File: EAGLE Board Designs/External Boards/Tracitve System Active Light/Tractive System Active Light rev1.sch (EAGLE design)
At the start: 25 parts, among them X1 CONNECTOR-4NANO-FIT-VERTICAL-4

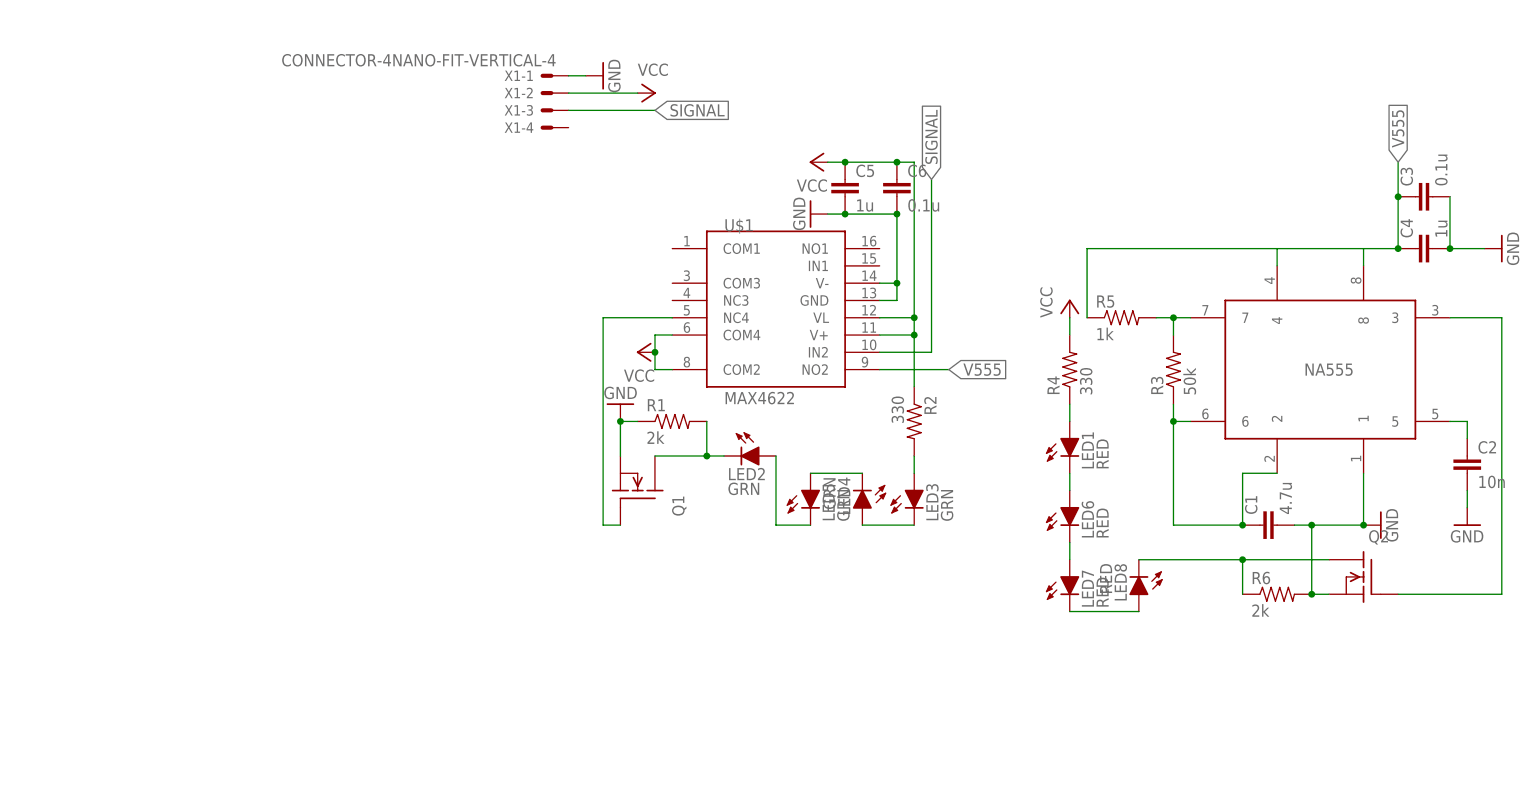
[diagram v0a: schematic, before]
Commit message: Later version of TSAL schematic and board
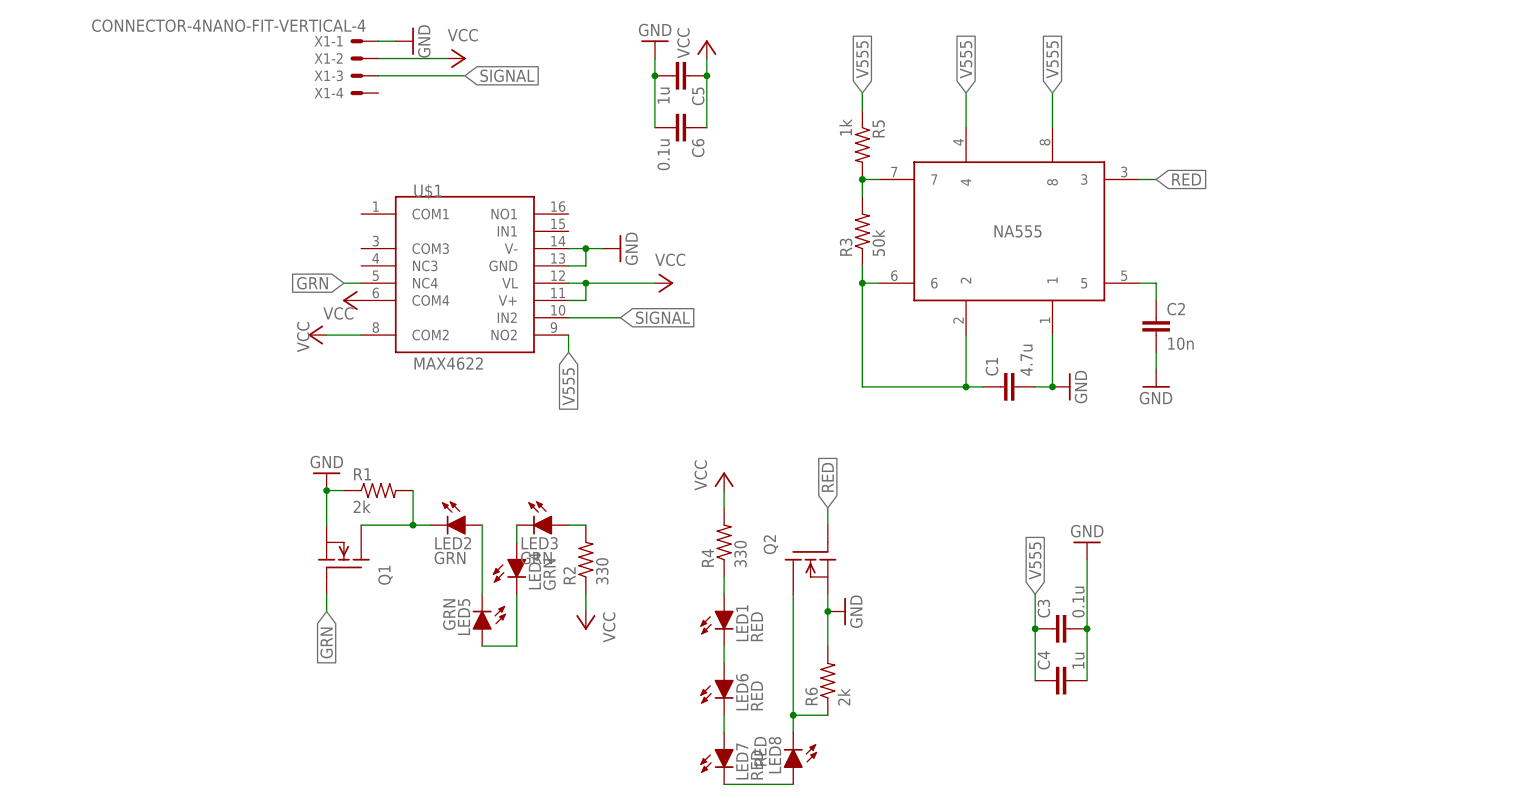
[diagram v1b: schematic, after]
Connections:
- net N$12 renamed RED
- net N$7 renamed GRN
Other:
- moved on the sheet: C1, C2, C3, C4, C5, C6, LED1, LED2, LED3, LED4, LED5, LED6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
